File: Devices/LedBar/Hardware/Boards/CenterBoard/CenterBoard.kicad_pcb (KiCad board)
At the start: 2 copper layers, 120 x 24 mm, 0 parts

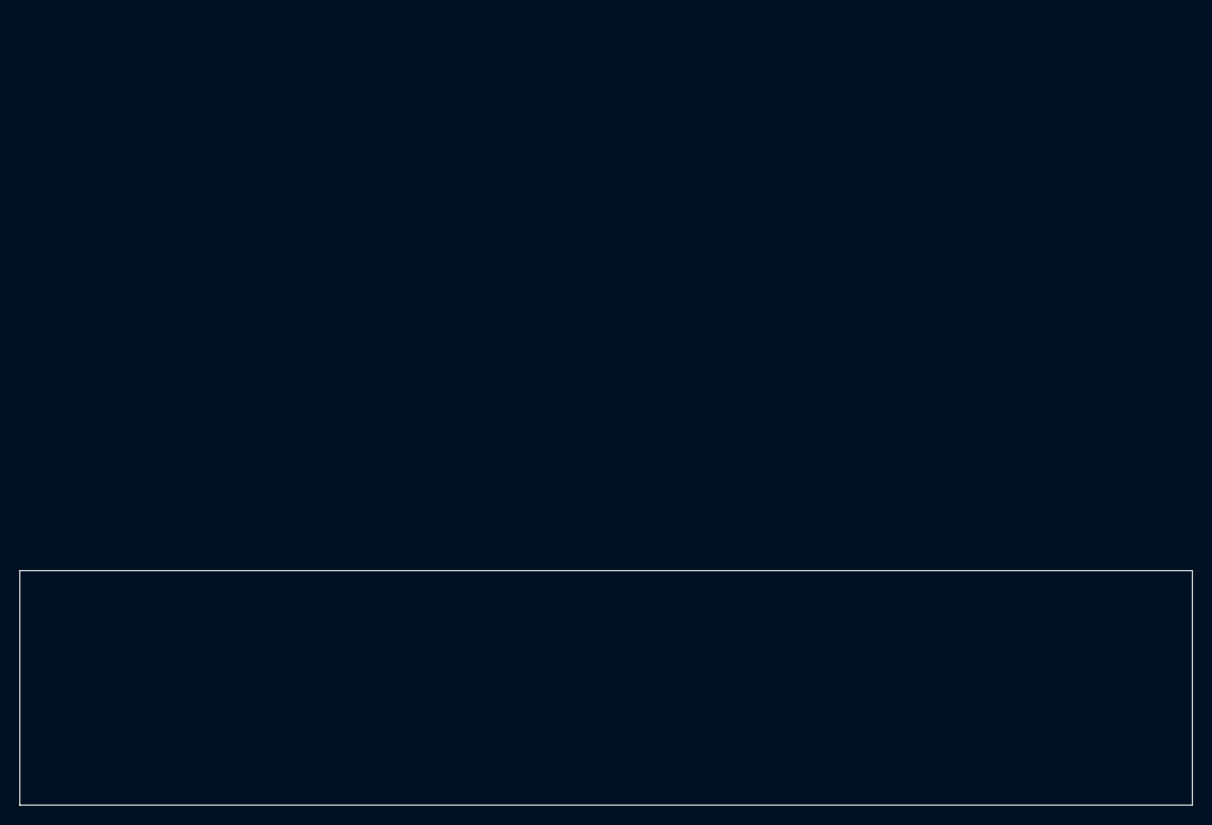
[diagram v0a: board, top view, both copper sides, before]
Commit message: Added PCA schematic
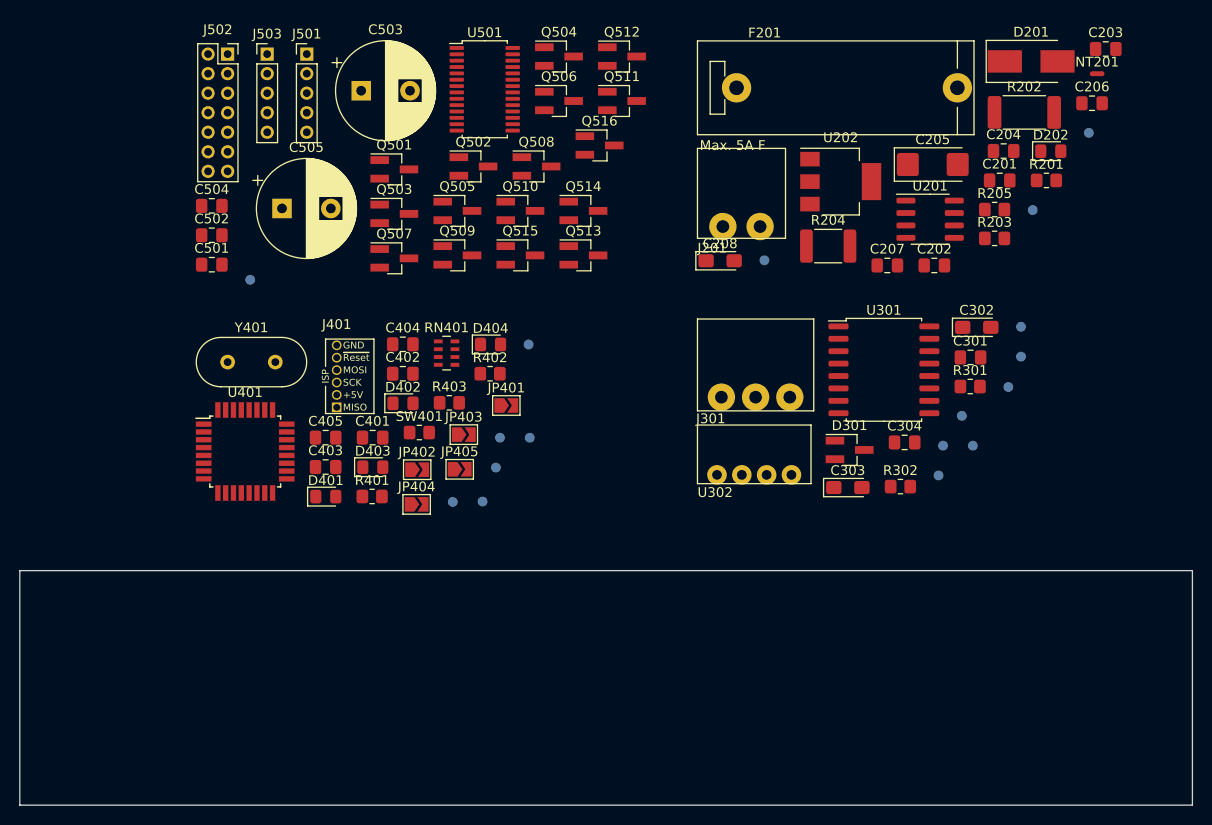
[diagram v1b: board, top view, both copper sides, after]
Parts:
- added C201: 0.1uF, Capacitor_SMD:C_0805_2012Metric_Pad1.18x1.45mm_HandSolder, F.Cu at (200.3, 60.1)
- added C202: 1uF, Capacitor_SMD:C_0805_2012Metric_Pad1.18x1.45mm_HandSolder, F.Cu at (193.6, 68.8)
- added C203: 0.1uF, Capacitor_SMD:C_0805_2012Metric_Pad1.18x1.45mm_HandSolder, F.Cu at (211.1, 46.6)
- added C204: 0.1uF, Capacitor_SMD:C_0805_2012Metric_Pad1.18x1.45mm_HandSolder, F.Cu at (200.7, 57.1)
- added C205: 10uF/16V, Capacitor_Tantalum_SMD:CP_EIA-6032-28_Kemet-C_Pad2.25x2.35mm_HandSolder, F.Cu at (193.4, 58.4)
- added C206: 0.1uF, Capacitor_SMD:C_0805_2012Metric_Pad1.18x1.45mm_HandSolder, F.Cu at (209.7, 52.2)
- added C207: 0.1uF, Capacitor_SMD:C_0805_2012Metric_Pad1.18x1.45mm_HandSolder, F.Cu at (188.8, 68.8)
- added C208: 10uF/10V, Capacitor_Tantalum_SMD:CP_EIA-3216-18_Kemet-A_Pad1.58x1.35mm_HandSolder, F.Cu at (171.7, 68.3)
- added C301: 0.1uF, Capacitor_SMD:C_0805_2012Metric_Pad1.18x1.45mm_HandSolder, F.Cu at (197.3, 78.2)
- added C302: 10uF, Capacitor_Tantalum_SMD:CP_EIA-3216-18_Kemet-A_Pad1.58x1.35mm_HandSolder, F.Cu at (197.9, 75.1)
- added C303: 4.7uF, Capacitor_Tantalum_SMD:CP_EIA-3216-18_Kemet-A_Pad1.58x1.35mm_HandSolder, F.Cu at (184.7, 91.5)
- added C304: 0.1uF, Capacitor_SMD:C_0805_2012Metric_Pad1.18x1.45mm_HandSolder, F.Cu at (190.5, 86.9)
- added C401: 0.1uF, Capacitor_SMD:C_0805_2012Metric_Pad1.18x1.45mm_HandSolder, F.Cu at (136.1, 86.4)
- added C402: 0.1uF, Capacitor_SMD:C_0805_2012Metric_Pad1.18x1.45mm_HandSolder, F.Cu at (139.2, 79.9)
- added C403: 0.1uF, Capacitor_SMD:C_0805_2012Metric_Pad1.18x1.45mm_HandSolder, F.Cu at (131.3, 89.4)
- added C404: 22pF, Capacitor_SMD:C_0805_2012Metric_Pad1.18x1.45mm_HandSolder, F.Cu at (139.2, 76.8)
- added C405: 22pF, Capacitor_SMD:C_0805_2012Metric_Pad1.18x1.45mm_HandSolder, F.Cu at (131.3, 86.4)
- added C501: 0.1uF, Capacitor_SMD:C_0805_2012Metric_Pad1.18x1.45mm_HandSolder, F.Cu at (119.6, 68.7)
- added C502: 0.1uF, Capacitor_SMD:C_0805_2012Metric_Pad1.18x1.45mm_HandSolder, F.Cu at (119.6, 65.7)
- added C503: 1000uF/16V, Capacitor_THT:CP_Radial_D10.0mm_P5.00mm, F.Cu at (134.9, 50.9)
- added C504: 0.1uF, Capacitor_SMD:C_0805_2012Metric_Pad1.18x1.45mm_HandSolder, F.Cu at (119.6, 62.7)
- added C505: 1000uF/16V, Capacitor_THT:CP_Radial_D10.0mm_P5.00mm, F.Cu at (126.8, 62.9)
- added D201: SMBJ15A, Diode_SMD:D_SMB_Handsoldering, F.Cu at (203.5, 47.9)
- added D202: Blue, LED_SMD:LED_0805_2012Metric_Pad1.15x1.40mm_HandSolder, F.Cu at (205.5, 57.1)
- added D301: PSM712, Package_TO_SOT_SMD:SOT-23_Handsoldering, F.Cu at (184.9, 87.7)
- added D401: Green, LED_SMD:LED_0805_2012Metric_Pad1.15x1.40mm_HandSolder, F.Cu at (131.3, 92.4)
- added D402: Yellow, LED_SMD:LED_0805_2012Metric_Pad1.15x1.40mm_HandSolder, F.Cu at (139.2, 82.9)
- added D403: Orange, LED_SMD:LED_0805_2012Metric_Pad1.15x1.40mm_HandSolder, F.Cu at (136.1, 89.4)
- added D404: Red, LED_SMD:LED_0805_2012Metric_Pad1.15x1.40mm_HandSolder, F.Cu at (148.2, 76.9)
- added F201: Max. 5A F, AmbientLight:Fuseholder_Cylinder-5x20mm_BLX_A_Horizontal, F.Cu at (173.3, 50.6)
- added J201: 12VDC/5A, AmbientLight:15EDGRC-3.81-2P, F.Cu at (171.9, 64.8)
- added J301: RS485, AmbientLight:15EDGRC-3.5-3P, F.Cu at (171.8, 82.3)
- added J401: AVR-ISP-6, AmbientLight:ISP_P1.27mm_single_row, F.Cu at (132.4, 76.9)
- added J501: Left, Connector_PinHeader_2.00mm:PinHeader_1x05_P2.00mm_Vertical, F.Cu at (129.4, 47.1)
- added J502: Center, Connector_PinSocket_2.00mm:PinSocket_2x07_P2.00mm_Vertical, F.Cu at (121.3, 47.1)
- added J503: Right, Connector_PinHeader_2.00mm:PinHeader_1x05_P2.00mm_Vertical, F.Cu at (125.3, 47.1)
- added JP401: SolderJumper_2_Open, Jumper:SolderJumper-2_P1.3mm_Open_TrianglePad1.0x1.5mm, F.Cu at (149.8, 83.1)
- added JP402: SolderJumper_2_Open, Jumper:SolderJumper-2_P1.3mm_Open_TrianglePad1.0x1.5mm, F.Cu at (140.7, 89.7)
- added JP403: SolderJumper_2_Open, Jumper:SolderJumper-2_P1.3mm_Open_TrianglePad1.0x1.5mm, F.Cu at (145.4, 86.1)
- added JP404: SolderJumper_2_Open, Jumper:SolderJumper-2_P1.3mm_Open_TrianglePad1.0x1.5mm, F.Cu at (140.6, 93.2)
- added JP405: SolderJumper_2_Open, Jumper:SolderJumper-2_P1.3mm_Open_TrianglePad1.0x1.5mm, F.Cu at (145.0, 89.6)
- added NT201: Net-Tie_2, NetTie:NetTie-2_SMD_Pad0.5mm, F.Cu at (210.2, 49.2)
- added Q501: Si2302DS, Package_TO_SOT_SMD:SOT-23_Handsoldering, F.Cu at (138.3, 58.9)
- added Q502: Si2302DS, Package_TO_SOT_SMD:SOT-23_Handsoldering, F.Cu at (146.4, 58.6)
- added Q503: Si2302DS, Package_TO_SOT_SMD:SOT-23_Handsoldering, F.Cu at (138.3, 63.5)
- added Q504: Si2302DS, Package_TO_SOT_SMD:SOT-23_Handsoldering, F.Cu at (155.2, 47.4)
- added Q505: Si2302DS, Package_TO_SOT_SMD:SOT-23_Handsoldering, F.Cu at (144.8, 63.2)
- added Q506: Si2302DS, Package_TO_SOT_SMD:SOT-23_Handsoldering, F.Cu at (155.2, 51.9)
- added Q507: Si2302DS, Package_TO_SOT_SMD:SOT-23_Handsoldering, F.Cu at (138.3, 68.0)
- added Q508: Si2302DS, Package_TO_SOT_SMD:SOT-23_Handsoldering, F.Cu at (152.9, 58.6)
- added Q509: Si2302DS, Package_TO_SOT_SMD:SOT-23_Handsoldering, F.Cu at (144.8, 67.7)
- added Q510: Si2302DS, Package_TO_SOT_SMD:SOT-23_Handsoldering, F.Cu at (151.2, 63.2)
- added Q511: Si2302DS, Package_TO_SOT_SMD:SOT-23_Handsoldering, F.Cu at (161.6, 51.9)
- added Q512: Si2302DS, Package_TO_SOT_SMD:SOT-23_Handsoldering, F.Cu at (161.6, 47.4)
- added Q513: Si2302DS, Package_TO_SOT_SMD:SOT-23_Handsoldering, F.Cu at (157.7, 67.7)
- added Q514: Si2302DS, Package_TO_SOT_SMD:SOT-23_Handsoldering, F.Cu at (157.7, 63.2)
- added Q515: Si2302DS, Package_TO_SOT_SMD:SOT-23_Handsoldering, F.Cu at (151.2, 67.7)
- added Q516: Si2302DS, Package_TO_SOT_SMD:SOT-23_Handsoldering, F.Cu at (159.3, 56.5)
- added R201: 10R, Resistor_SMD:R_0805_2012Metric_Pad1.20x1.40mm_HandSolder, F.Cu at (205.1, 60.1)
- added R202: R001/2W, Resistor_SMD:R_2512_6332Metric_Pad1.40x3.35mm_HandSolder, F.Cu at (202.8, 53.1)
- added R203: 10R, Resistor_SMD:R_0805_2012Metric_Pad1.20x1.40mm_HandSolder, F.Cu at (199.8, 66.0)
- added R204: 100R/1W, Resistor_SMD:R_1812_4532Metric_Pad1.30x3.40mm_HandSolder, F.Cu at (182.7, 66.8)
- added R205: 10k, Resistor_SMD:R_0805_2012Metric_Pad1.20x1.40mm_HandSolder, F.Cu at (199.8, 63.1)
- added R301: 120, Resistor_SMD:R_0805_2012Metric_Pad1.20x1.40mm_HandSolder, F.Cu at (197.3, 81.2)
- added R302: 120, Resistor_SMD:R_0805_2012Metric_Pad1.20x1.40mm_HandSolder, F.Cu at (190.1, 91.4)
- added R401: 4k7, Resistor_SMD:R_0805_2012Metric_Pad1.20x1.40mm_HandSolder, F.Cu at (136.1, 92.4)
- added R402: 10k, Resistor_SMD:R_0805_2012Metric_Pad1.20x1.40mm_HandSolder, F.Cu at (148.1, 79.9)
- added R403: 4k7, Resistor_SMD:R_0805_2012Metric_Pad1.20x1.40mm_HandSolder, F.Cu at (144.0, 82.8)
- added RN401: 10k, Resistor_SMD:R_Array_Concave_4x0603, F.Cu at (143.7, 77.7)
- added SW401: reset, Resistor_SMD:R_0805_2012Metric_Pad1.20x1.40mm_HandSolder, F.Cu at (140.9, 85.9)
- added TP201: gnd, AmbientLight:TestPoint_Pad_D1.0mm, F.Cu at (203.7, 63.1)
- added TP202: +12V, AmbientLight:TestPoint_Pad_D1.0mm, F.Cu at (209.4, 55.2)
- added TP203: +5V, AmbientLight:TestPoint_Pad_D1.0mm, F.Cu at (176.2, 68.2)
- added TP301: B, AmbientLight:TestPoint_Pad_D1.0mm, F.Cu at (197.5, 87.2)
- added TP302: A, AmbientLight:TestPoint_Pad_D1.0mm, F.Cu at (202.5, 78.1)
- added TP303: +5V_iso, AmbientLight:TestPoint_Pad_D1.0mm, F.Cu at (196.4, 84.2)
- added TP304: GND_iso, AmbientLight:TestPoint_Pad_D1.0mm, F.Cu at (202.5, 75.1)
- added TP305: txd, AmbientLight:TestPoint_Pad_D1.0mm, F.Cu at (194.0, 90.3)
- added TP306: rxd, AmbientLight:TestPoint_Pad_D1.0mm, F.Cu at (201.2, 81.2)
- added TP307: tx_en, AmbientLight:TestPoint_Pad_D1.0mm, F.Cu at (194.5, 87.2)
- added TP401: dbg1, AmbientLight:TestPoint_Pad_D1.0mm, F.Cu at (152.1, 76.9)
- added TP402: dbg2, AmbientLight:TestPoint_Pad_D1.0mm, F.Cu at (149.1, 86.4)
- added TP403: scl, AmbientLight:TestPoint_Pad_D1.0mm, F.Cu at (144.3, 93.0)
- added TP404: ~reset~, AmbientLight:TestPoint_Pad_D1.0mm, F.Cu at (148.7, 89.5)
- added TP405: ~button~, AmbientLight:TestPoint_Pad_D1.0mm, F.Cu at (152.2, 86.4)
- added TP406: sda, AmbientLight:TestPoint_Pad_D1.0mm, F.Cu at (147.4, 92.9)
- added TP501: ~pca_oe~, AmbientLight:TestPoint_Pad_D1.0mm, F.Cu at (123.6, 70.2)
- added U201: INA219AxD, Package_SO:SOIC-8_3.9x4.9mm_P1.27mm, F.Cu at (193.2, 64.0)
- added U202: AMS1117-5.0, Package_TO_SOT_SMD:SOT-223-3_TabPin2, F.Cu at (184.0, 60.2)
- added U301: ISO3082DW, Package_SO:SOIC-16W_7.5x10.3mm_P1.27mm, F.Cu at (188.4, 79.5)
- added U302: B0505S-1W-SIP4, AmbientLight:B0505S-1W, F.Cu at (171.3, 90.2)
- added U401: ATmega48PV-10AU-arduino, Package_QFP:TQFP-32_7x7mm_P0.8mm, F.Cu at (123.1, 87.8)
- added U501: PCA9685PW, Package_SO:TSSOP-28_4.4x9.7mm_P0.65mm, F.Cu at (147.6, 50.7)
- added Y401: 14.7456Mhz, Crystal:Crystal_HC49-U_Vertical, F.Cu at (121.3, 78.7)

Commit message: Added 0-10V schematic
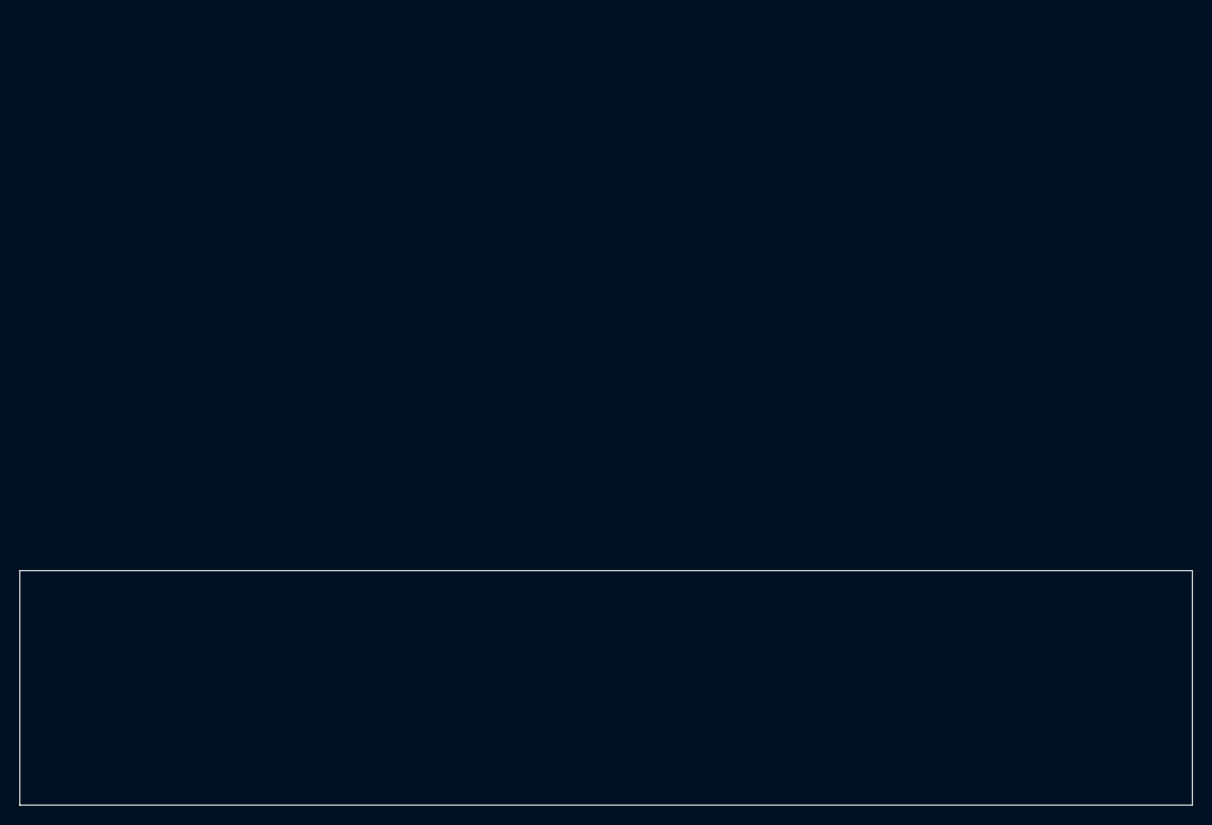
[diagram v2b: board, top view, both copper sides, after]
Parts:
- removed C201, C203, C204, C206, C207, C301, C304, C401, C402, C403, C501, C502, C504: 0.1uF, Capacitor_SMD:C_0805_2012Metric_Pad1.18x1.45mm_HandSolder
- removed C202: 1uF, Capacitor_SMD:C_0805_2012Metric_Pad1.18x1.45mm_HandSolder
- removed C205: 10uF/16V, Capacitor_Tantalum_SMD:CP_EIA-6032-28_Kemet-C_Pad2.25x2.35mm_HandSolder
- removed C208: 10uF/10V, Capacitor_Tantalum_SMD:CP_EIA-3216-18_Kemet-A_Pad1.58x1.35mm_HandSolder
- removed C302: 10uF, Capacitor_Tantalum_SMD:CP_EIA-3216-18_Kemet-A_Pad1.58x1.35mm_HandSolder
- removed C303: 4.7uF, Capacitor_Tantalum_SMD:CP_EIA-3216-18_Kemet-A_Pad1.58x1.35mm_HandSolder
- removed C404, C405: 22pF, Capacitor_SMD:C_0805_2012Metric_Pad1.18x1.45mm_HandSolder
- removed C503, C505: 1000uF/16V, Capacitor_THT:CP_Radial_D10.0mm_P5.00mm
- removed D201: SMBJ15A, Diode_SMD:D_SMB_Handsoldering
- removed D202: Blue, LED_SMD:LED_0805_2012Metric_Pad1.15x1.40mm_HandSolder
- removed D301: PSM712, Package_TO_SOT_SMD:SOT-23_Handsoldering
- removed D401: Green, LED_SMD:LED_0805_2012Metric_Pad1.15x1.40mm_HandSolder
- removed D402: Yellow, LED_SMD:LED_0805_2012Metric_Pad1.15x1.40mm_HandSolder
- removed D403: Orange, LED_SMD:LED_0805_2012Metric_Pad1.15x1.40mm_HandSolder
- removed D404: Red, LED_SMD:LED_0805_2012Metric_Pad1.15x1.40mm_HandSolder
- removed F201: Max. 5A F, AmbientLight:Fuseholder_Cylinder-5x20mm_BLX_A_Horizontal
- removed J201: 12VDC/5A, AmbientLight:15EDGRC-3.81-2P
- removed J301: RS485, AmbientLight:15EDGRC-3.5-3P
- removed J401: AVR-ISP-6, AmbientLight:ISP_P1.27mm_single_row
- removed J501: Left, Connector_PinHeader_2.00mm:PinHeader_1x05_P2.00mm_Vertical
- removed J502: Center, Connector_PinSocket_2.00mm:PinSocket_2x07_P2.00mm_Vertical
- removed J503: Right, Connector_PinHeader_2.00mm:PinHeader_1x05_P2.00mm_Vertical
- removed JP401, JP402, JP403, JP404, JP405: SolderJumper_2_Open, Jumper:SolderJumper-2_P1.3mm_Open_TrianglePad1.0x1.5mm
- removed NT201: Net-Tie_2, NetTie:NetTie-2_SMD_Pad0.5mm
- removed Q501, Q502, Q503, Q504, Q505, Q506, Q507, Q508, Q509, Q510, Q511, Q512, Q513, Q514, Q515, Q516: Si2302DS, Package_TO_SOT_SMD:SOT-23_Handsoldering
- removed R201, R203: 10R, Resistor_SMD:R_0805_2012Metric_Pad1.20x1.40mm_HandSolder
- removed R202: R001/2W, Resistor_SMD:R_2512_6332Metric_Pad1.40x3.35mm_HandSolder
- removed R204: 100R/1W, Resistor_SMD:R_1812_4532Metric_Pad1.30x3.40mm_HandSolder
- removed R205, R402: 10k, Resistor_SMD:R_0805_2012Metric_Pad1.20x1.40mm_HandSolder
- removed R301, R302: 120, Resistor_SMD:R_0805_2012Metric_Pad1.20x1.40mm_HandSolder
- removed R401, R403: 4k7, Resistor_SMD:R_0805_2012Metric_Pad1.20x1.40mm_HandSolder
- removed RN401: 10k, Resistor_SMD:R_Array_Concave_4x0603
- removed SW401: reset, Resistor_SMD:R_0805_2012Metric_Pad1.20x1.40mm_HandSolder
- removed TP201: gnd, AmbientLight:TestPoint_Pad_D1.0mm
- removed TP202: +12V, AmbientLight:TestPoint_Pad_D1.0mm
- removed TP203: +5V, AmbientLight:TestPoint_Pad_D1.0mm
- removed TP301: B, AmbientLight:TestPoint_Pad_D1.0mm
- removed TP302: A, AmbientLight:TestPoint_Pad_D1.0mm
- removed TP303: +5V_iso, AmbientLight:TestPoint_Pad_D1.0mm
- removed TP304: GND_iso, AmbientLight:TestPoint_Pad_D1.0mm
- removed TP305: txd, AmbientLight:TestPoint_Pad_D1.0mm
- removed TP306: rxd, AmbientLight:TestPoint_Pad_D1.0mm
- removed TP307: tx_en, AmbientLight:TestPoint_Pad_D1.0mm
- removed TP401: dbg1, AmbientLight:TestPoint_Pad_D1.0mm
- removed TP402: dbg2, AmbientLight:TestPoint_Pad_D1.0mm
- removed TP403: scl, AmbientLight:TestPoint_Pad_D1.0mm
- removed TP404: ~reset~, AmbientLight:TestPoint_Pad_D1.0mm
- removed TP405: ~button~, AmbientLight:TestPoint_Pad_D1.0mm
- removed TP406: sda, AmbientLight:TestPoint_Pad_D1.0mm
- removed TP501: ~pca_oe~, AmbientLight:TestPoint_Pad_D1.0mm
- removed U201: INA219AxD, Package_SO:SOIC-8_3.9x4.9mm_P1.27mm
- removed U202: AMS1117-5.0, Package_TO_SOT_SMD:SOT-223-3_TabPin2
- removed U301: ISO3082DW, Package_SO:SOIC-16W_7.5x10.3mm_P1.27mm
- removed U302: B0505S-1W-SIP4, AmbientLight:B0505S-1W
- removed U401: ATmega48PV-10AU-arduino, Package_QFP:TQFP-32_7x7mm_P0.8mm
- removed U501: PCA9685PW, Package_SO:TSSOP-28_4.4x9.7mm_P0.65mm
- removed Y401: 14.7456Mhz, Crystal:Crystal_HC49-U_Vertical
